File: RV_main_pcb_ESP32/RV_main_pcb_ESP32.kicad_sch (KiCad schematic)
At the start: 55 parts, among them J1 Conn_01x07_Female, J2 Conn_01x03_Female, J3 Conn_01x02_Male, J4 Conn_01x02_Male, J5 Conn_02x03_Top_Bottom, Q1 AO3400A, Q2 AO3401A, U1 ESP32_DevKit_V1_DOIT, U2 LM1117-5, U3 TXS0102DCT, U4 INA226, U5 LM1117-5

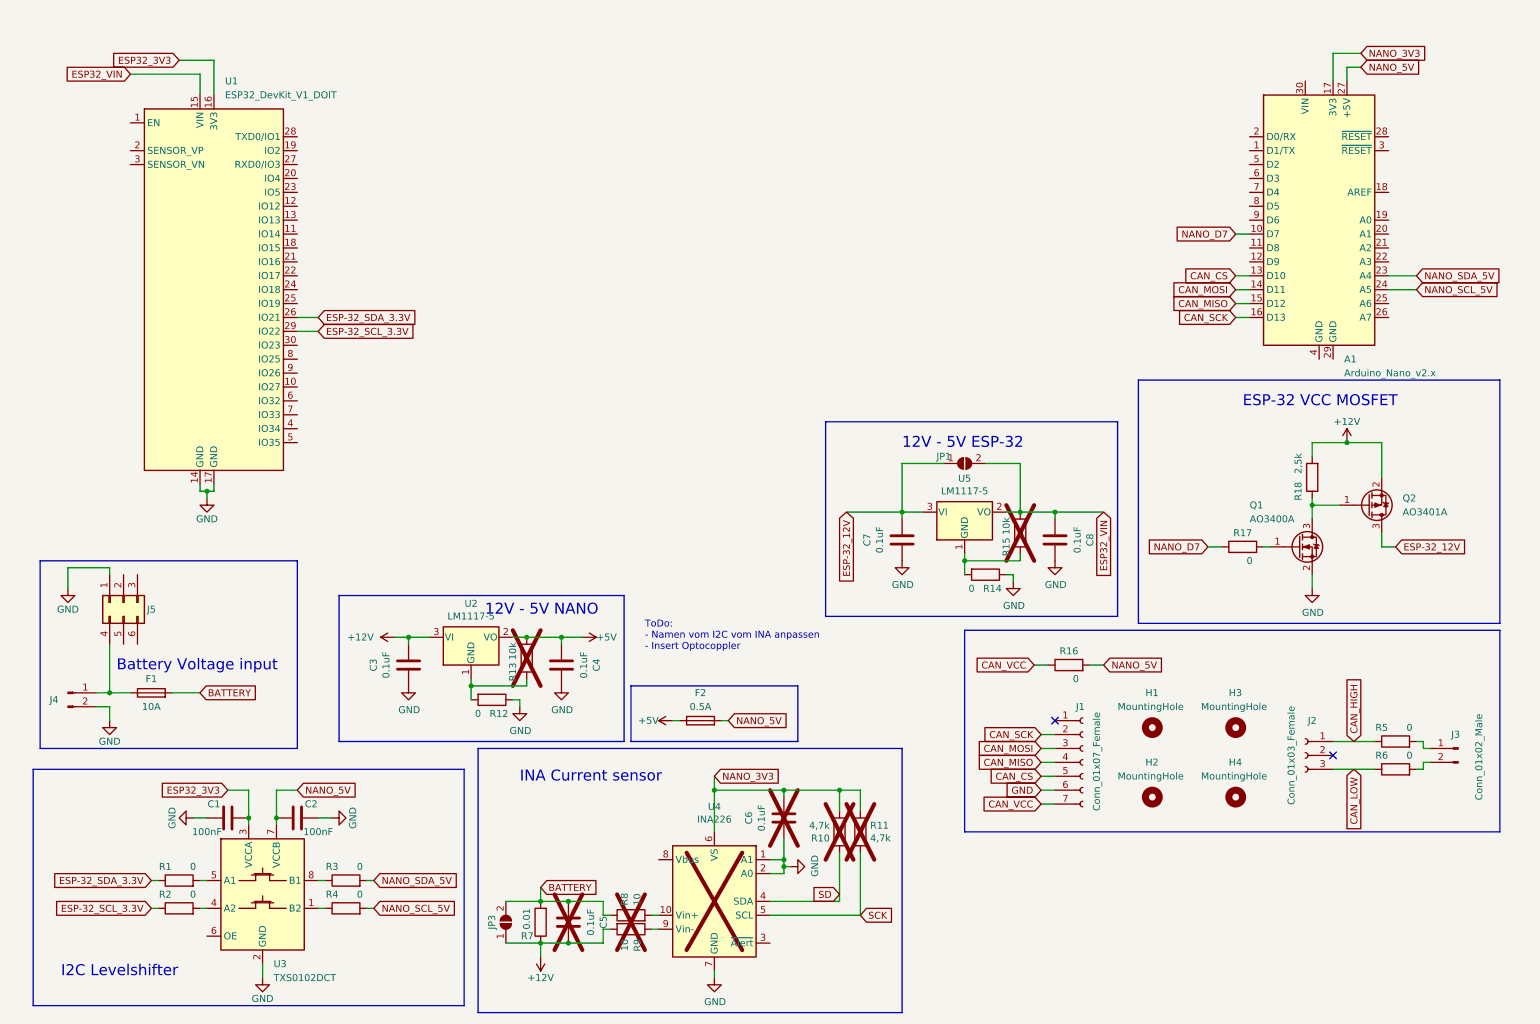
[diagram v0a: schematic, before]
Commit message: update
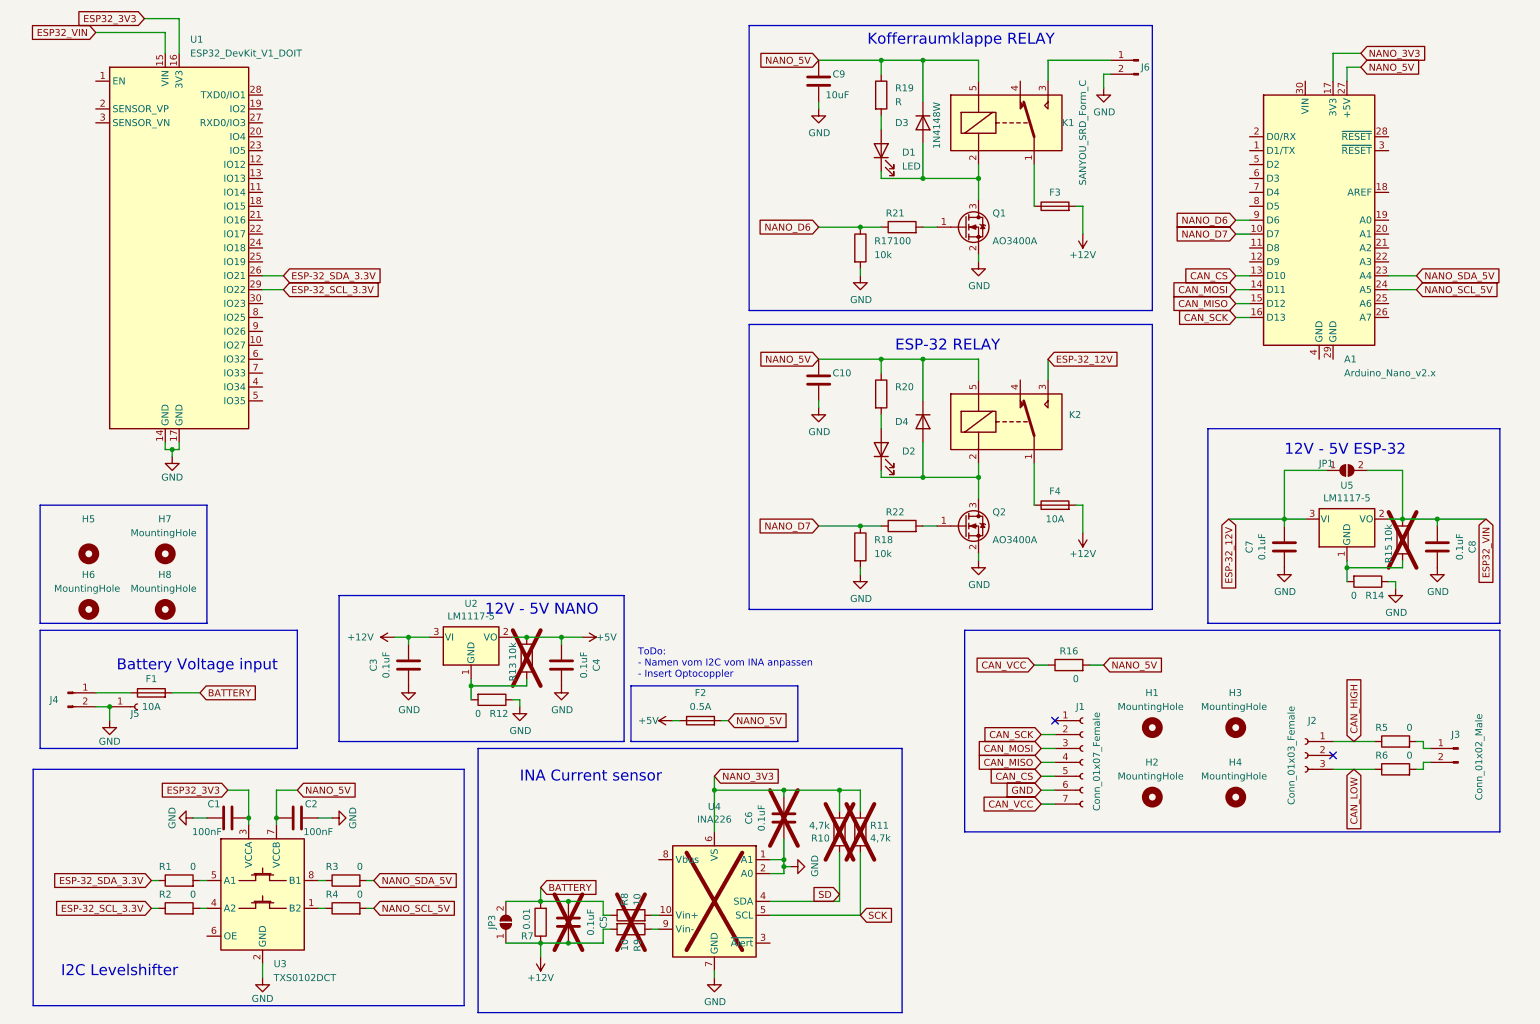
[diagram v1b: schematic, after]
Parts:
- removed J5: Conn_02x03_Top_Bottom, Connector_Molex:Molex_Mini-Fit_Jr_5569-06A2_2x03_P4.20mm_Horizontal, symbol Connector_Generic:Conn_02x03_Top_Bottom
- removed Q2: AO3401A, Package_TO_SOT_SMD:SOT-23, symbol Transistor_FET:AO3401A
- added C10: (no value), symbol Device:C
- added C9: 10uF, Capacitor_SMD:C_0603_1608Metric, symbol Device:C
- added D1: LED, symbol Device:LED
- added D2: (no value), symbol Device:LED
- added D3: 1N4148W, Diode_SMD:D_SOD-123, symbol Diode:1N4148W
- added D4: (no value), symbol Diode:1N4148W
- added F3: (no value), symbol Device:Fuse
- added F4: 10A, symbol Device:Fuse
- added H5: (no value), symbol Mechanical:MountingHole
- added H6, H7, H8: MountingHole, MountingHole:MountingHole_4.3mm_M4_DIN965, symbol Mechanical:MountingHole
- added J5: (no value), symbol Connector:Conn_01x01_Female
- added J6: (no value), symbol Connector:Conn_01x02_Male
- added K1: SANYOU_SRD_Form_C, Relay_THT:Relay_SPDT_SANYOU_SRD_Series_Form_C, symbol Relay:SANYOU_SRD_Form_C
- added K2: (no value), symbol Relay:SANYOU_SRD_Form_C
- added Q2: AO3400A, Package_TO_SOT_SMD:SOT-23, symbol Transistor_FET:AO3400A
- added R19: R, symbol Device:R
- added R20, R22: (no value), symbol Device:R
- added R21: 100, symbol Device:R
- J4: value Conn_01x02_Male -> (none); footprint TerminalBlock:TerminalBlock_bornier-2_P5.08mm -> (none)
- R17: value 0 -> 10k; footprint Resistor_SMD:R_0805_2012Metric -> (none)
- R18: value 2,5k -> 10k; footprint Resistor_SMD:R_0603_1608Metric -> (none)
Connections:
- net +12V: now also F3.2, F4.2; no longer R18.2
- net ESP-32_12V: now also K2.3
- net GND: now also R17.2, R18.2, C10.2, C9.2, J5.1 (Pin_1), J6.2 (Pin_2), Q2.2 (S)
- net NANO_5V: now also C10.1, C9.1, D3.1 (K), D4.1 (K), K1.5, K2.5, R19.1, R20.1
- net NANO_D7: now also R18.1, R22.1; no longer R17.1
- net at Q1.1 (G): now also R21.2; no longer R17.2
- net at Q1.3 (D): now also D1.1 (K), D3.2 (A), K1.2; no longer R18.1
- net NANO_D6: now reaches A1.9 (D6)
- net NANO_D6: now also R17.1, R21.1
- new net: F3.1, K1.1
- new net: J6.1 (Pin_1), K1.3
- new net: D1.2 (A), R19.2
- new net: Q2.1 (G), R22.2
- new net: F4.1, K2.1
- new net: D2.1 (K), D4.2 (A), K2.2, Q2.3 (D)
- new net: D2.2 (A), R20.2
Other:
- note added: "ESP-32 RELAY"
- note added: "Kofferraumklappe RELAY"
- note removed: "ESP-32 VCC MOSFET"
- moved on the sheet: C7, C8, JP1, R14, R15, U1, U5

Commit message: update
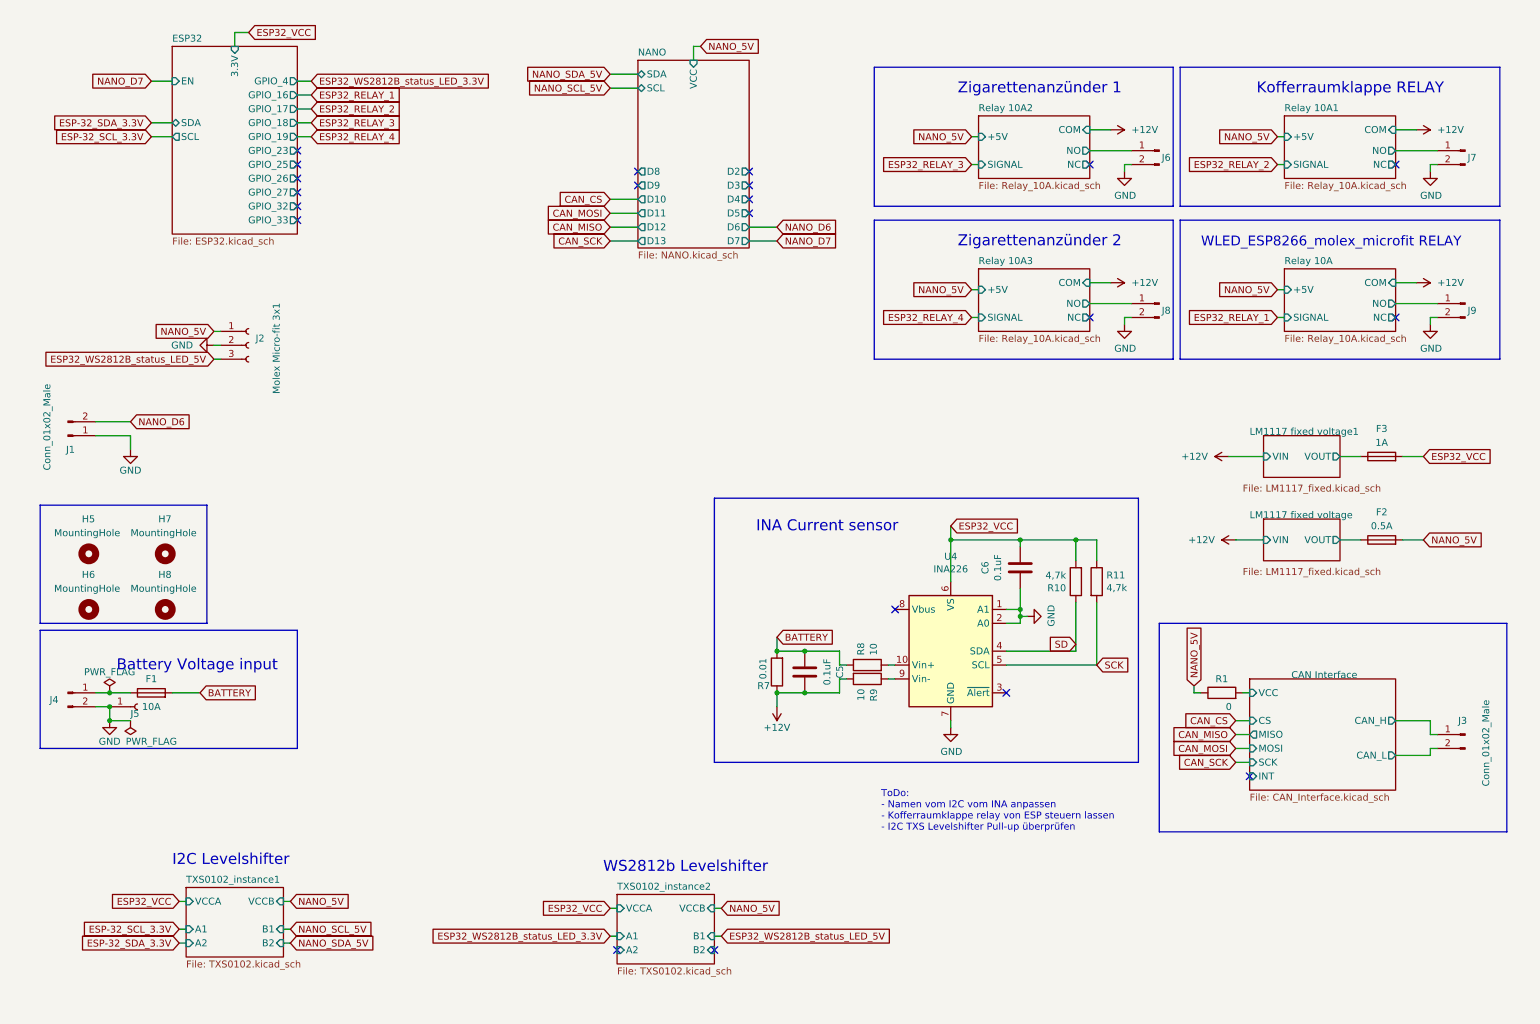
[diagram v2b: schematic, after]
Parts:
- removed A1: Arduino_Nano_v2.x, Module:Arduino_Nano, symbol MCU_Module:Arduino_Nano_v2.x
- removed C1, C2: 100nF, Capacitor_SMD:C_0402_1005Metric, symbol Device:C
- removed C10: (no value), symbol Device:C
- removed C3, C4, C7, C8: 0.1uF, Capacitor_SMD:C_0805_2012Metric, symbol Device:C
- removed C9: 10uF, Capacitor_SMD:C_0603_1608Metric, symbol Device:C
- removed D1: LED, symbol Device:LED
- removed D2: (no value), symbol Device:LED
- removed D3: 1N4148W, Diode_SMD:D_SOD-123, symbol Diode:1N4148W
- removed D4: (no value), symbol Diode:1N4148W
- removed DNP1, DNP2, DNP3, DNP5, DNP6, DNP7, DNP8: DNP_small, symbol Fabian_Barth:DNP_small
- removed DNP4: DNP_large, symbol Fabian_Barth:DNP_large
- removed F4: 10A, symbol Device:Fuse
- removed H1, H2, H3, H4: MountingHole, MountingHole:MountingHole_3.2mm_M3_ISO7380, symbol Mechanical:MountingHole
- removed J1: Conn_01x07_Female, Connector_PinHeader_2.54mm:PinHeader_1x06_P2.54mm_Vertical, symbol Connector:Conn_01x07_Female
- removed JP1, JP3: SolderJumper_2_Open, Jumper:SolderJumper-2_P1.3mm_Open_RoundedPad1.0x1.5mm, symbol Jumper:SolderJumper_2_Open
- removed K1: SANYOU_SRD_Form_C, Relay_THT:Relay_SPDT_SANYOU_SRD_Series_Form_C, symbol Relay:SANYOU_SRD_Form_C
- removed K2: (no value), symbol Relay:SANYOU_SRD_Form_C
- removed Q1, Q2: AO3400A, Package_TO_SOT_SMD:SOT-23, symbol Transistor_FET:AO3400A
- removed R12, R14, R16: 0, Resistor_SMD:R_0805_2012Metric, symbol Device:R
- removed R13, R15: 10k, Resistor_SMD:R_0805_2012Metric, symbol Device:R
- removed R17, R18: 10k, symbol Device:R
- removed R19: R, symbol Device:R
- removed R2, R3, R4: 0, Resistor_SMD:R_1206_3216Metric, symbol Device:R
- removed R20, R22: (no value), symbol Device:R
- removed R21: 100, symbol Device:R
- removed R5, R6: 0, Resistor_SMD:R_0603_1608Metric, symbol Device:R
- removed U1: ESP32_DevKit_V1_DOIT, esp32_devkit_v1_doit:esp32_devkit_v1_doit, symbol esp32_devkit_v1_doit:ESP32_DevKit_V1_DOIT
- removed U2, U5: LM1117-5, Package_TO_SOT_SMD:SOT-223, symbol Regulator_Linear:LM1117-3.3
- removed U3: TXS0102DCT, Package_SO:SSOP-8_2.95x2.8mm_P0.65mm, symbol Logic_LevelTranslator:TXS0102DCT
- added J1: Conn_01x02_Male, Connector_Molex:Molex_Micro-Fit_3.0_43650-0200_1x02_P3.00mm_Horizontal, symbol Connector:Conn_01x02_Male
- added J7, J8, J9: Conn_01x02_Male, TerminalBlock:TerminalBlock_bornier-2_P5.08mm, symbol Connector:Conn_01x02_Male
- F1: footprint (none) -> custom_librarys:Flachsicherung
- F3: value (none) -> 1A; footprint (none) -> Fuse:Fuse_1206_3216Metric
- H5: value (none) -> MountingHole; footprint (none) -> MountingHole:MountingHole_3.2mm_M3
- H6, H7, H8: footprint MountingHole:MountingHole_4.3mm_M4_DIN965 -> MountingHole:MountingHole_3.2mm_M3
- J2: value Conn_01x03_Female -> Molex Micro-fit 3x1; footprint Connector_PinHeader_2.54mm:PinHeader_1x03_P2.54mm_Vertical -> Connector_Molex:Molex_Micro-Fit_3.0_43650-0300_1x03_P3.00mm_Horizontal
- J4, J6: value (none) -> Conn_01x02_Male; footprint (none) -> TerminalBlock:TerminalBlock_bornier-2_P5.08mm
- J5: value (none) -> Conn_01x01_Female; footprint (none) -> Connector:Banana_Jack_1Pin
- R1: footprint Resistor_SMD:R_1206_3216Metric -> Resistor_SMD:R_0805_2012Metric
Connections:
- net CAN_HIGH is gone; now on net NANO_5V: J2.1 (Pin_1)
- net +12V: no longer F3.2
- net ESP-32_SDA_3.3V: no longer R1.1
- net GND: now also J2.2 (Pin_2), J1.1 (Pin_1), J7.2 (Pin_2), J8.2 (Pin_2), J9.2 (Pin_2)
- net NANO_5V: now also R1.1
- net NANO_D6: now also J1.2 (Pin_2)
- net LM1117 fixed voltage1/VOUT: now reaches F3.1
- net Relay 10A2/NO: now reaches J6.1 (Pin_1)
- net CAN Interface/VCC: now reaches R1.2
- net CAN Interface/CAN_H: now reaches J3.1 (Pin_1)
- net CAN Interface/CAN_L: now reaches J3.2 (Pin_2)
- net +5V renamed LM1117 fixed voltage/VOUT
- net CAN_LOW renamed ESP32_WS2812B_status_LED_5V
- net NANO_3V3 renamed ESP32_VCC
- net ESP32_VCC: now also F3.2
- new net Relay 10A/NO: J9.1 (Pin_1)
- new net Relay 10A1/NO: J7.1 (Pin_1)
- new net Relay 10A3/NO: J8.1 (Pin_1)
- no-connect marks 2 -> 21
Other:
- added sheet CAN Interface (CAN_Interface.kicad_sch)
- added sheet ESP32 (ESP32.kicad_sch)
- added sheet LM1117 fixed voltage (LM1117_fixed.kicad_sch)
- added sheet LM1117 fixed voltage1 (LM1117_fixed.kicad_sch)
- added sheet NANO (NANO.kicad_sch)
- added sheet Relay 10A (Relay_10A.kicad_sch)
- added sheet Relay 10A1 (Relay_10A.kicad_sch)
- added sheet Relay 10A2 (Relay_10A.kicad_sch)
- added sheet Relay 10A3 (Relay_10A.kicad_sch)
- added sheet TXS0102_instance1 (TXS0102.kicad_sch)
- added sheet TXS0102_instance2 (TXS0102.kicad_sch)
- note added: "ToDo: - Namen vom I2C vom INA anpassen - Kofferraumklappe relay von ESP steuern lassen - I2C TXS Levelshifter Pull-up überprüfen"
- note added: "WLED_ESP8266_molex_microfit RELAY"
- note added: "WS2812b Levelshifter"
- note added: "Zigarettenanzünder 1"
- note added: "Zigarettenanzünder 2"
- note removed: "12V - 5V ESP-32"
- note removed: "12V - 5V NANO"
- note removed: "ESP-32 RELAY"
- note removed: "ToDo: - Namen vom I2C vom INA anpassen - Insert Optocoppler"
- moved on the sheet: C5, C6, J3, R10, R11, R7, R8, R9, U4
